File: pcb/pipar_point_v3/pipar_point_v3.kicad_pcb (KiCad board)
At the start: 4 copper layers, 353 parts, among them IC1 MCP1700T-3302E_MAY, IC2 MCP1700T-3302E_MAY, J1 USB_C_Receptacle_USB2.0_16P, J2 USB_C_Receptacle_USB2.0_16P, J3 Conn_02x03_Odd_Even, J4 Conn_02x03_Odd_Even, Q1 AO3400A, Q2 AO3400A, SW1 EVP-BB1AAB000, SW2 EVP-BB1AAB000, SW3 SW_SPDT, SW4 SW_SPDT, U1 ISP1807-LR-RS, U2 ISP1807-LR-RS, U3 MAX17048, U4 ESDR0502NMUTAG, U5 nPM1100-QDXX, U6 MAX17048, U7 ESDR0502NMUTAG, U8 nPM1100-QDXX

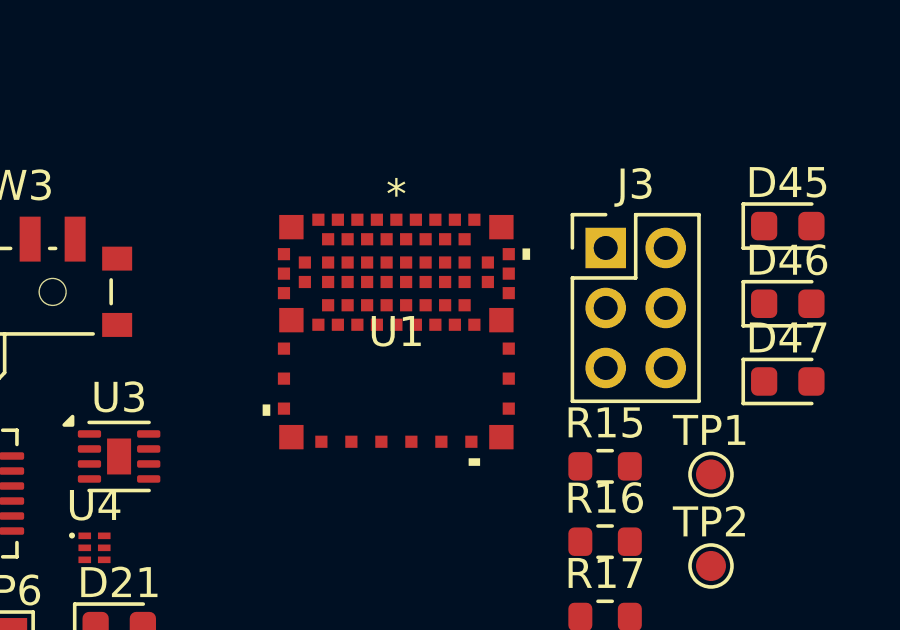
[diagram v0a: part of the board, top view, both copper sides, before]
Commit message: updates the pinout for the isp1807
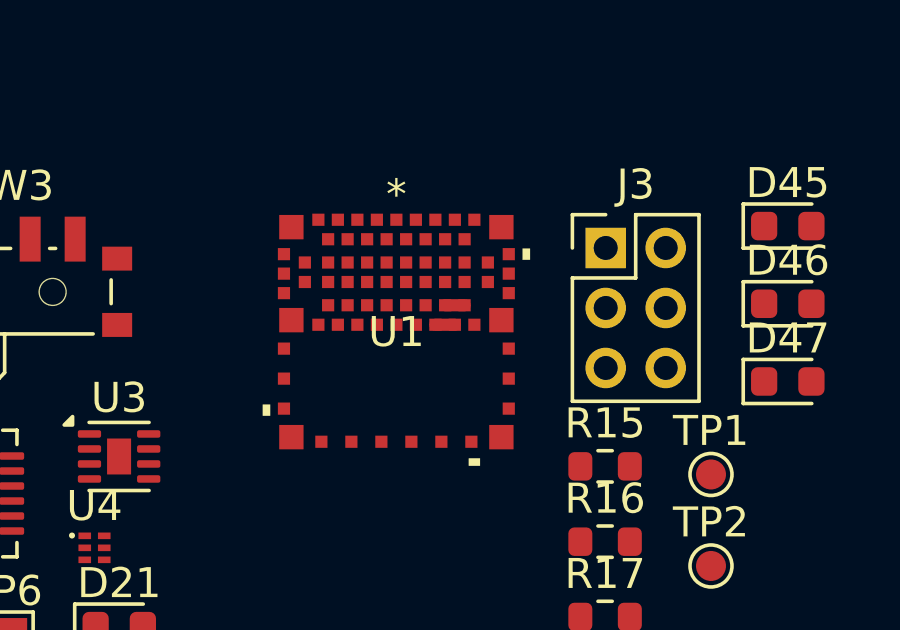
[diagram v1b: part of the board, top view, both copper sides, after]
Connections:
- U1 pad 32: unconnected-(U1A-P0_08-Pad32) -> /Side-Left/BAT_SDA
- U1 pad 34: unconnected-(U1A-P0_06-Pad34) -> /Side-Left/BAT_SCL
- U1 pad 36: unconnected-(U1A-P0_05_AIN3-Pad36) -> /Side-Left/Col6
- U1 pad 38: unconnected-(U1A-P0_03_AIN1-Pad38) -> /Side-Left/Col5
- U1 pad 40: unconnected-(U1A-P0_02_AIN0-Pad40) -> /Side-Left/Col4
- U1 pad 42: unconnected-(U1A-P0_31_AIN7-Pad42) -> /Side-Left/Col3
- U1 pad 44: unconnected-(U1A-P0_30_AIN6-Pad44) -> /Side-Left/Col2
- U1 pad 46: unconnected-(U1A-P0_29_AIN5-Pad46) -> /Side-Left/Col1
- U1 pad 48: unconnected-(U1A-P0_28_AIN4-Pad48) -> /Side-Left/Col0
- U1 pad 50: unconnected-(U1A-P1_06-Pad50) -> /Side-Left/LED_3
- U1 pad 52: unconnected-(U1A-P1_14-Pad52) -> /Side-Left/LED_1
- U1 pad 54: unconnected-(U1A-P1_05-Pad54) -> /Side-Left/Row2
- U1 pad 56: unconnected-(U1A-P1_09_TRACEDATA3-Pad56) -> /Side-Left/Row0
- U1 pad 59: unconnected-(U1A-P1_12-Pad59) -> /Side-Left/LED_2
- U1 pad 61: unconnected-(U1A-P1_11-Pad61) -> /Side-Left/Backlight
- U1 pad 63: unconnected-(U1A-P1_04-Pad63) -> /Side-Left/Row1
- U2 pad 32: unconnected-(U2A-P0_08-Pad32) -> /Side-Right/BAT_SDA
- U2 pad 34: unconnected-(U2A-P0_06-Pad34) -> /Side-Right/BAT_SCL
- U2 pad 36: unconnected-(U2A-P0_05_AIN3-Pad36) -> /Side-Right/Col6
- U2 pad 38: unconnected-(U2A-P0_03_AIN1-Pad38) -> /Side-Right/Col5
- U2 pad 40: unconnected-(U2A-P0_02_AIN0-Pad40) -> /Side-Right/Col4
- U2 pad 42: unconnected-(U2A-P0_31_AIN7-Pad42) -> /Side-Right/Col3
- U2 pad 44: unconnected-(U2A-P0_30_AIN6-Pad44) -> /Side-Right/Col2
- U2 pad 46: unconnected-(U2A-P0_29_AIN5-Pad46) -> /Side-Right/Col1
- U2 pad 48: unconnected-(U2A-P0_28_AIN4-Pad48) -> /Side-Right/Col0
- U2 pad 50: unconnected-(U2A-P1_06-Pad50) -> /Side-Right/LED_3
- U2 pad 52: unconnected-(U2A-P1_14-Pad52) -> /Side-Right/LED_1
- U2 pad 54: unconnected-(U2A-P1_05-Pad54) -> /Side-Right/Row2
- U2 pad 56: unconnected-(U2A-P1_09_TRACEDATA3-Pad56) -> /Side-Right/Row0
- U2 pad 59: unconnected-(U2A-P1_12-Pad59) -> /Side-Right/LED_2
- U2 pad 61: unconnected-(U2A-P1_11-Pad61) -> /Side-Right/Backlight
- U2 pad 63: unconnected-(U2A-P1_04-Pad63) -> /Side-Right/Row1
- U4 pad 2: unconnected-(U4-NC-Pad2) -> /Side-Left/USB_D+
- U4 pad 3: unconnected-(U4-NC-Pad3) -> /Side-Left/USB_D-
- U7 pad 2: unconnected-(U7-NC-Pad2) -> /Side-Right/USB_D+
- U7 pad 3: unconnected-(U7-NC-Pad3) -> /Side-Right/USB_D-
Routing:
- net GND: track 0.00 -> 0.65 mm
- net Net-(U1A-OUT_ANT): track 0.00 -> 0.65 mm

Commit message: Place keys on the left hand side
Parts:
- added D54: D_Small, Diode_SMD:D_SOD-523, B.Cu at (303.3, 107.0)
- added D55: D_Small, Diode_SMD:D_SOD-523, B.Cu at (317.7, 95.0)
- added D56: D_Small, Diode_SMD:D_SOD-523, B.Cu at (333.1, 84.4)
- added D57: D_Small, Diode_SMD:D_SOD-523, B.Cu at (325.8, 55.4)
- added D58: D_Small, Diode_SMD:D_SOD-523, B.Cu at (324.3, 38.5)
- added D59: D_Small, Diode_SMD:D_SOD-523, B.Cu at (322.8, 21.7)
- added D60: D_Small, Diode_SMD:D_SOD-523, B.Cu at (344.5, 50.3)
- added D61: D_Small, Diode_SMD:D_SOD-523, B.Cu at (343.1, 33.4)
- added D62: D_Small, Diode_SMD:D_SOD-523, B.Cu at (341.6, 16.5)
- added D63: D_Small, Diode_SMD:D_SOD-523, B.Cu at (364.2, 47.2)
- added D64: D_Small, Diode_SMD:D_SOD-523, B.Cu at (364.2, 30.2)
- added D65: D_Small, Diode_SMD:D_SOD-523, B.Cu at (364.2, 13.3)
- added D66: D_Small, Diode_SMD:D_SOD-523, B.Cu at (383.7, 52.4)
- added D67: D_Small, Diode_SMD:D_SOD-523, B.Cu at (385.2, 35.5)
- added D68: D_Small, Diode_SMD:D_SOD-523, B.Cu at (386.7, 18.6)
- added D69: D_Small, Diode_SMD:D_SOD-523, B.Cu at (401.0, 68.6)
- added D70: D_Small, Diode_SMD:D_SOD-523, B.Cu at (408.1, 53.2)
- added D71: D_Small, Diode_SMD:D_SOD-523, B.Cu at (415.3, 37.8)
- added D72: D_Small, Diode_SMD:D_SOD-523, B.Cu at (419.5, 72.1)
- added D73: D_Small, Diode_SMD:D_SOD-523, B.Cu at (426.7, 56.7)
- added H72: SwitchHoles, Keyboard:SwitchHoles_Kailh_Choc_V1V2, F.Cu at (309.7, 101.7)
- added H73: SwitchHoles, Keyboard:SwitchHoles_Kailh_Choc_V1V2, F.Cu at (324.5, 90.3)
- added H74: SwitchHoles, Keyboard:SwitchHoles_Kailh_Choc_V1V2, F.Cu at (340.3, 80.2)
- added H75: SwitchHoles, Keyboard:SwitchHoles_Kailh_Choc_V1V2, F.Cu at (334.1, 54.6)
- added H76: SwitchHoles, Keyboard:SwitchHoles_Kailh_Choc_V1V2, F.Cu at (332.6, 37.8)
- added H77: SwitchHoles, Keyboard:SwitchHoles_Kailh_Choc_V1V2, F.Cu at (331.1, 20.9)
- added H78: SwitchHoles, Keyboard:SwitchHoles_Kailh_Choc_V1V2, F.Cu at (352.8, 49.5)
- added H79: SwitchHoles, Keyboard:SwitchHoles_Kailh_Choc_V1V2, F.Cu at (351.3, 32.7)
- added H80: SwitchHoles, Keyboard:SwitchHoles_Kailh_Choc_V1V2, F.Cu at (349.8, 15.8)
- added H81: SwitchHoles, Keyboard:SwitchHoles_Kailh_Choc_V1V2, F.Cu at (372.5, 47.2)
- added H82: SwitchHoles, Keyboard:SwitchHoles_Kailh_Choc_V1V2, F.Cu at (372.5, 30.2)
- added H83: SwitchHoles, Keyboard:SwitchHoles_Kailh_Choc_V1V2, F.Cu at (372.5, 13.3)
- added H84: SwitchHoles, Keyboard:SwitchHoles_Kailh_Choc_V1V2, F.Cu at (392.0, 53.1)
- added H85: SwitchHoles, Keyboard:SwitchHoles_Kailh_Choc_V1V2, F.Cu at (393.5, 36.2)
- added H86: SwitchHoles, Keyboard:SwitchHoles_Kailh_Choc_V1V2, F.Cu at (394.9, 19.3)
- added H87: SwitchHoles, Keyboard:SwitchHoles_Kailh_Choc_V1V2, F.Cu at (408.5, 72.1)
- added H88: SwitchHoles, Keyboard:SwitchHoles_Kailh_Choc_V1V2, F.Cu at (415.6, 56.7)
- added H89: SwitchHoles, Keyboard:SwitchHoles_Kailh_Choc_V1V2, F.Cu at (422.8, 41.3)
- added H90: SwitchHoles, Keyboard:SwitchHoles_Kailh_Choc_V1V2, F.Cu at (427.0, 75.6)
- added H91: SwitchHoles, Keyboard:SwitchHoles_Kailh_Choc_V1V2, F.Cu at (434.2, 60.2)
- added KHS50: KHS, Keyboard:Kailh_HS_Socket, F.Cu at (310.9, 107.0)
- added KHS51: KHS, Keyboard:Kailh_HS_Socket, F.Cu at (325.3, 95.7)
- added KHS52: KHS, Keyboard:Kailh_HS_Socket, F.Cu at (340.6, 85.7)
- added KHS53: KHS, Keyboard:Kailh_HS_Socket, F.Cu at (332.0, 59.7)
- added KHS54: KHS, Keyboard:Kailh_HS_Socket, F.Cu at (330.5, 42.9)
- added KHS55: KHS, Keyboard:Kailh_HS_Socket, F.Cu at (329.0, 26.0)
- added KHS56: KHS, Keyboard:Kailh_HS_Socket, F.Cu at (350.7, 54.6)
- added KHS57: KHS, Keyboard:Kailh_HS_Socket, F.Cu at (349.2, 37.8)
- added KHS58: KHS, Keyboard:Kailh_HS_Socket, F.Cu at (347.8, 20.9)
- added KHS59: KHS, Keyboard:Kailh_HS_Socket, F.Cu at (370.0, 52.1)
- added KHS60: KHS, Keyboard:Kailh_HS_Socket, F.Cu at (370.0, 35.1)
- added KHS61: KHS, Keyboard:Kailh_HS_Socket, F.Cu at (370.0, 18.2)
- added KHS62: KHS, Keyboard:Kailh_HS_Socket, F.Cu at (389.1, 57.8)
- added KHS63: KHS, Keyboard:Kailh_HS_Socket, F.Cu at (390.5, 40.9)
- added KHS64: KHS, Keyboard:Kailh_HS_Socket, F.Cu at (392.0, 24.0)
- added KHS65: KHS, Keyboard:Kailh_HS_Socket, F.Cu at (404.1, 75.4)
- added KHS66: KHS, Keyboard:Kailh_HS_Socket, F.Cu at (411.3, 60.1)
- added KHS67: KHS, Keyboard:Kailh_HS_Socket, F.Cu at (418.5, 44.7)
- added KHS68: KHS, Keyboard:Kailh_HS_Socket, F.Cu at (422.7, 79.0)
- added KHS69: KHS, Keyboard:Kailh_HS_Socket, F.Cu at (429.9, 63.6)
- added LED50: LED_Small, LED_SMD:LED_0603_1608Metric, F.Cu at (306.4, 97.6)
- added LED51: LED_Small, LED_SMD:LED_0603_1608Metric, F.Cu at (321.6, 85.9)
- added LED52: LED_Small, LED_SMD:LED_0603_1608Metric, F.Cu at (337.8, 75.6)
- added LED53: LED_Small, LED_SMD:LED_0603_1608Metric, F.Cu at (333.7, 49.4)
- added LED54: LED_Small, LED_SMD:LED_0603_1608Metric, F.Cu at (332.1, 32.6)
- added LED55: LED_Small, LED_SMD:LED_0603_1608Metric, F.Cu at (330.6, 15.7)
- added LED56: LED_Small, LED_SMD:LED_0603_1608Metric, F.Cu at (352.3, 44.3)
- added LED57: LED_Small, LED_SMD:LED_0603_1608Metric, F.Cu at (351.0, 27.5)
- added LED58: LED_Small, LED_SMD:LED_0603_1608Metric, F.Cu at (349.4, 10.6)
- added LED59: LED_Small, LED_SMD:LED_0603_1608Metric, F.Cu at (372.5, 42.0)
- added LED60: LED_Small, LED_SMD:LED_0603_1608Metric, F.Cu at (372.5, 25.0)
- added LED61: LED_Small, LED_SMD:LED_0603_1608Metric, F.Cu at (372.5, 8.03)
- added LED62: LED_Small, LED_SMD:LED_0603_1608Metric, F.Cu at (392.4, 47.9)
- added LED63: LED_Small, LED_SMD:LED_0603_1608Metric, F.Cu at (393.9, 31.0)
- added LED64: LED_Small, LED_SMD:LED_0603_1608Metric, F.Cu at (395.4, 14.1)
- added LED65: LED_Small, LED_SMD:LED_0603_1608Metric, F.Cu at (410.7, 67.3)
- added LED66: LED_Small, LED_SMD:LED_0603_1608Metric, F.Cu at (417.9, 51.9)
- added LED67: LED_Small, LED_SMD:LED_0603_1608Metric, F.Cu at (425.0, 36.5)
- added LED68: LED_Small, LED_SMD:LED_0603_1608Metric, F.Cu at (429.3, 70.8)
- added LED69: LED_Small, LED_SMD:LED_0603_1608Metric, F.Cu at (436.4, 55.4)
- added LR50: R_Small, Resistor_SMD:R_0402_1005Metric, F.Cu at (307.2, 98.6)
- added LR51: R_Small, Resistor_SMD:R_0402_1005Metric, F.Cu at (322.3, 87.0)
- added LR52: R_Small, Resistor_SMD:R_0402_1005Metric, F.Cu at (338.4, 76.8)
- added LR53: R_Small, Resistor_SMD:R_0402_1005Metric, F.Cu at (333.8, 50.4)
- added LR54: R_Small, Resistor_SMD:R_0402_1005Metric, F.Cu at (332.2, 33.6)
- added LR55: R_Small, Resistor_SMD:R_0402_1005Metric, F.Cu at (330.7, 16.7)
- added LR56: R_Small, Resistor_SMD:R_0402_1005Metric, F.Cu at (352.4, 45.3)
- added LR57: R_Small, Resistor_SMD:R_0402_1005Metric, F.Cu at (351.1, 28.5)
- added LR58: R_Small, Resistor_SMD:R_0402_1005Metric, F.Cu at (349.5, 11.6)
- added LR59: R_Small, Resistor_SMD:R_0402_1005Metric, F.Cu at (372.5, 43.3)
- added LR60: R_Small, Resistor_SMD:R_0402_1005Metric, F.Cu at (372.4, 26.3)
- added LR61: R_Small, Resistor_SMD:R_0402_1005Metric, F.Cu at (372.5, 9.33)
- added LR62: R_Small, Resistor_SMD:R_0402_1005Metric, F.Cu at (392.3, 49.2)
- added LR63: R_Small, Resistor_SMD:R_0402_1005Metric, F.Cu at (393.8, 32.3)
- added LR64: R_Small, Resistor_SMD:R_0402_1005Metric, F.Cu at (395.3, 15.4)
- added LR65: R_Small, Resistor_SMD:R_0402_1005Metric, F.Cu at (410.1, 68.5)
- added LR66: R_Small, Resistor_SMD:R_0402_1005Metric, F.Cu at (417.3, 53.1)
- added LR67: R_Small, Resistor_SMD:R_0402_1005Metric, F.Cu at (424.5, 37.7)
- added LR68: R_Small, Resistor_SMD:R_0402_1005Metric, F.Cu at (428.7, 72.0)
- added LR69: R_Small, Resistor_SMD:R_0402_1005Metric, F.Cu at (435.9, 56.6)
- added U52: ~, Trackpoint:Trackpointer_4pin, B.Cu at (430.5, 44.8)
- added U53: ~, Trackpoint:Trackpoint_T460s_Stick, F.Cu at (408.9, 34.7)
- moved D4 166.7 mm to (88.6, -64.3), turned to -95 degrees
- moved LED4 166.2 mm to (97.6, -68.7), turned to -5 degrees
- moved KHS4 166.1 mm to (94.1, -58.9), turned to -5 degrees
- moved H4 166.0 mm to (97.1, -63.6), turned to -5 degrees
- moved LED16 155.7 mm to (3.27, -48.1), turned to 25 degrees
- moved H16 154.9 mm to (5.38, -43.4), turned to 25 degrees
- moved KHS16 153.2 mm to (5.19, -37.9), turned to 25 degrees
- moved D16 151.4 mm to (-2.35, -39.8), turned to -65 degrees
- moved LED19 148.1 mm to (-8.14, -29.2), turned to 25 degrees
- moved H19 146.7 mm to (-6.03, -24.5), turned to 25 degrees
- moved KHS19 144.5 mm to (-6.22, -19.0), turned to 25 degrees
- moved LED20 144.3 mm to (-0.97, -13.9), turned to 25 degrees
- moved D19 143.7 mm to (-13.8, -20.9), turned to -65 degrees
- moved D8 143.6 mm to (68.4, -52.5), turned to -95 degrees
- moved H20 143.0 mm to (1.14, -9.11), turned to 25 degrees
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
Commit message: Right hand side keys
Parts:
- moved LED24 152.9 mm to (170.1, -68.4), turned to 5 degrees
- moved H24 152.9 mm to (170.5, -63.2), turned to 5 degrees
- moved KHS24 152.6 mm to (168.4, -58.1), turned to 5 degrees
- moved D28 152.1 mm to (162.0, -62.5), turned to -85 degrees
- moved LED28 141.1 mm to (190.4, -56.6), turned to 5 degrees
- moved H28 141.0 mm to (190.7, -51.4), turned to 5 degrees
- moved KHS28 140.8 mm to (188.7, -46.3), turned to 5 degrees
- moved D32 140.3 mm to (182.2, -50.7), turned to -85 degrees
- moved LED27 140.2 mm to (188.9, -73.5), turned to 5 degrees
- moved H27 140.2 mm to (189.2, -68.3), turned to 5 degrees
- moved KHS27 139.9 mm to (187.2, -63.2), turned to 5 degrees
- moved D31 139.4 mm to (180.7, -67.6), turned to -85 degrees
- moved D40 136.2 mm to (254.4, -46.2), turned to -115 degrees
- moved KHS36 133.8 mm to (257.8, -39.2), turned to -25 degrees
- moved H36 132.5 mm to (262.2, -42.6), turned to -25 degrees
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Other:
- board outline added: 155.1 x 111.8 mm
